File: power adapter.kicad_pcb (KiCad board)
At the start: 2 copper layers, 76.2 x 50.8 mm, 0 parts

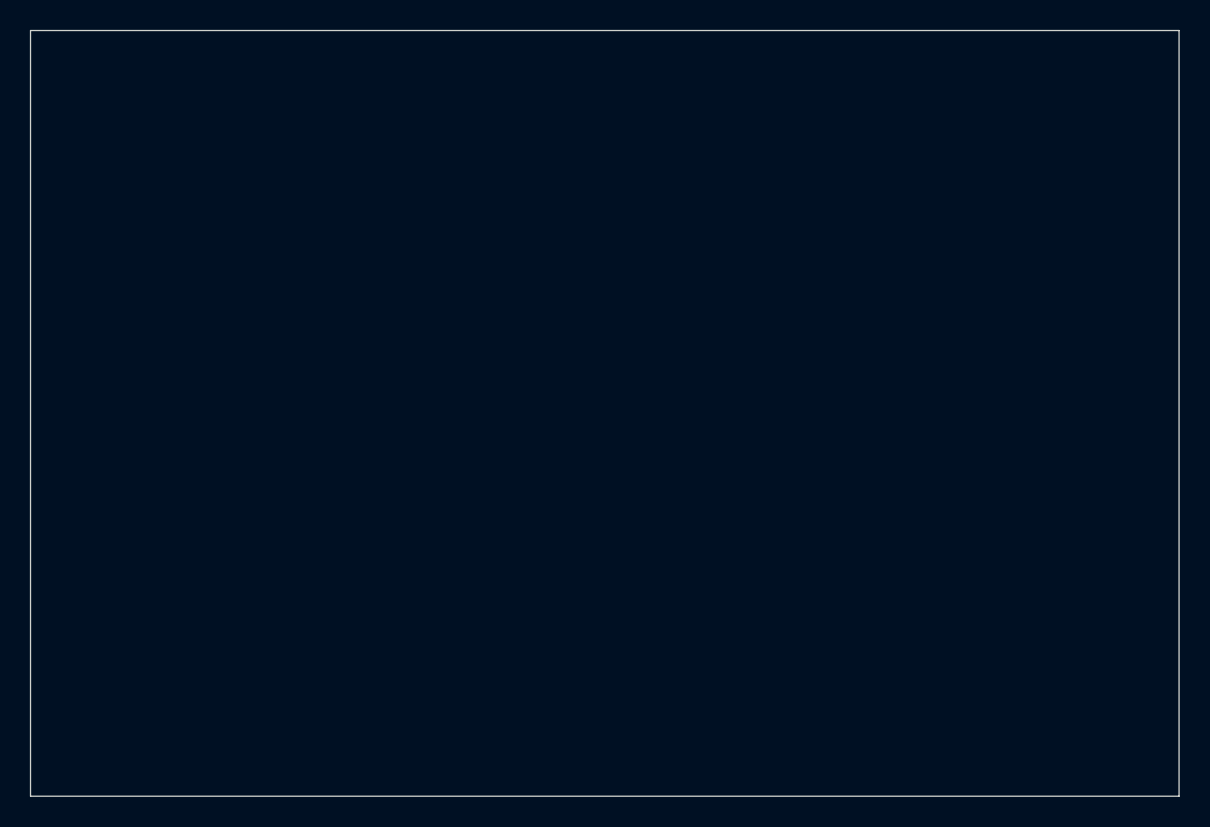
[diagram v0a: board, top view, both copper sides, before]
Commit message: board started
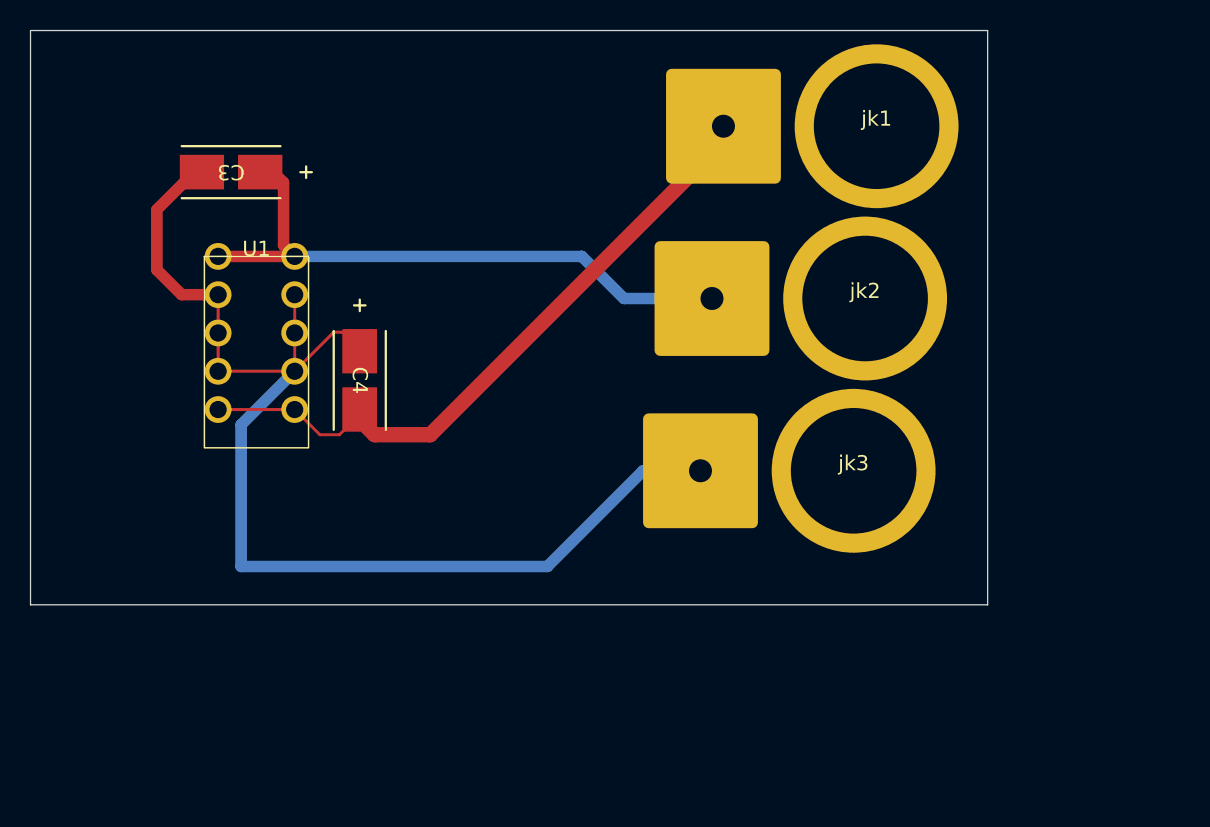
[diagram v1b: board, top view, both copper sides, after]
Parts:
- added C3: T491C106M025AT7280, customfootprints:10uFtantcap, F.Cu at (38.7, 85.6)
- added C4: T491C106M025AT7280, customfootprints:10uFtantcap, F.Cu at (47.2, 99.4)
- added U1: ~, adapterpcblib:Header2x5, F.Cu at (40.4, 91.2)
- added jk1: ~, adapterpcblib:Banana, F.Cu at (81.5, 82.5)
- added jk2: ~, adapterpcblib:Banana, F.Cu at (80.8, 94.0)
- added jk3: ~, adapterpcblib:Banana, F.Cu at (80.0, 105.4)
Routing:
- net GND: track 0.00 -> 81.5 mm
- net -12V: track 0.00 -> 45.3 mm
- net +12V: track 0.00 -> 41.3 mm
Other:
- board size 76.2 x 50.8 mm -> 63.5 x 38.1 mm
